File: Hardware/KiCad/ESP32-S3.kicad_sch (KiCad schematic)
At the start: 32 parts, among them J1 UJ20-C-H-G-SMT-1-P16-TR, J4 RJ45, J5 Conn_TagConnect_TC2030-NL_ESP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, U1 ESP32-S3-WROOM-1, U5 WE-TVS-82400102, U7 AP7333-33SRG-7

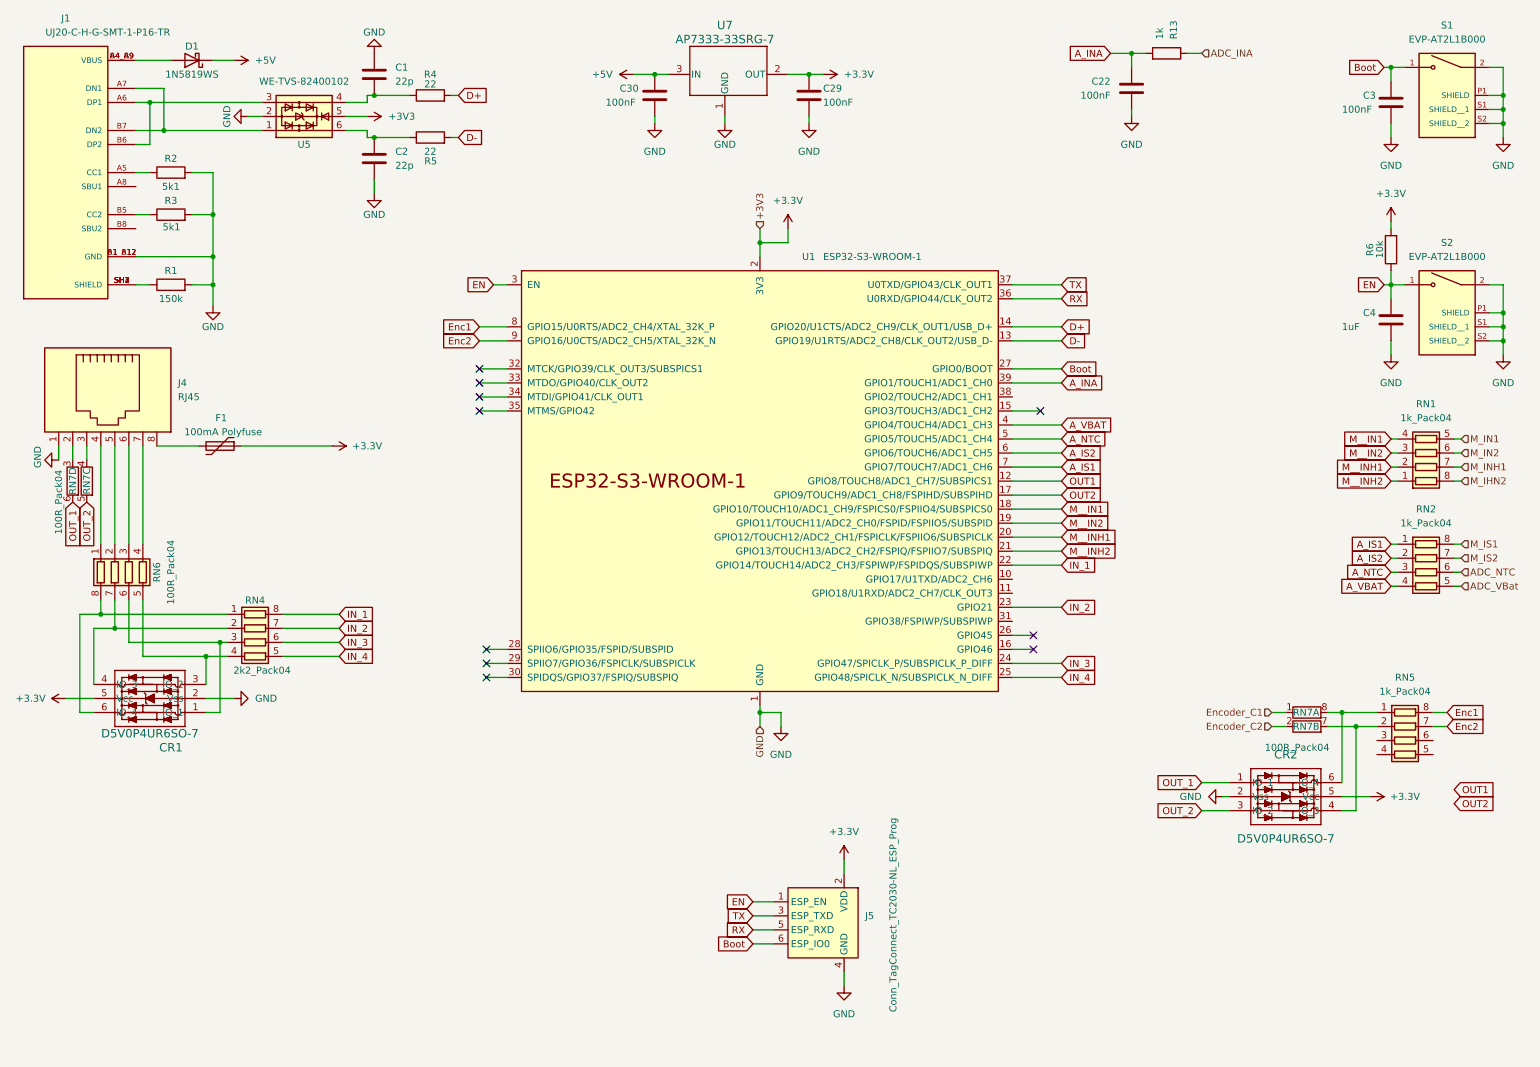
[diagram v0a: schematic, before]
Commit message: routing
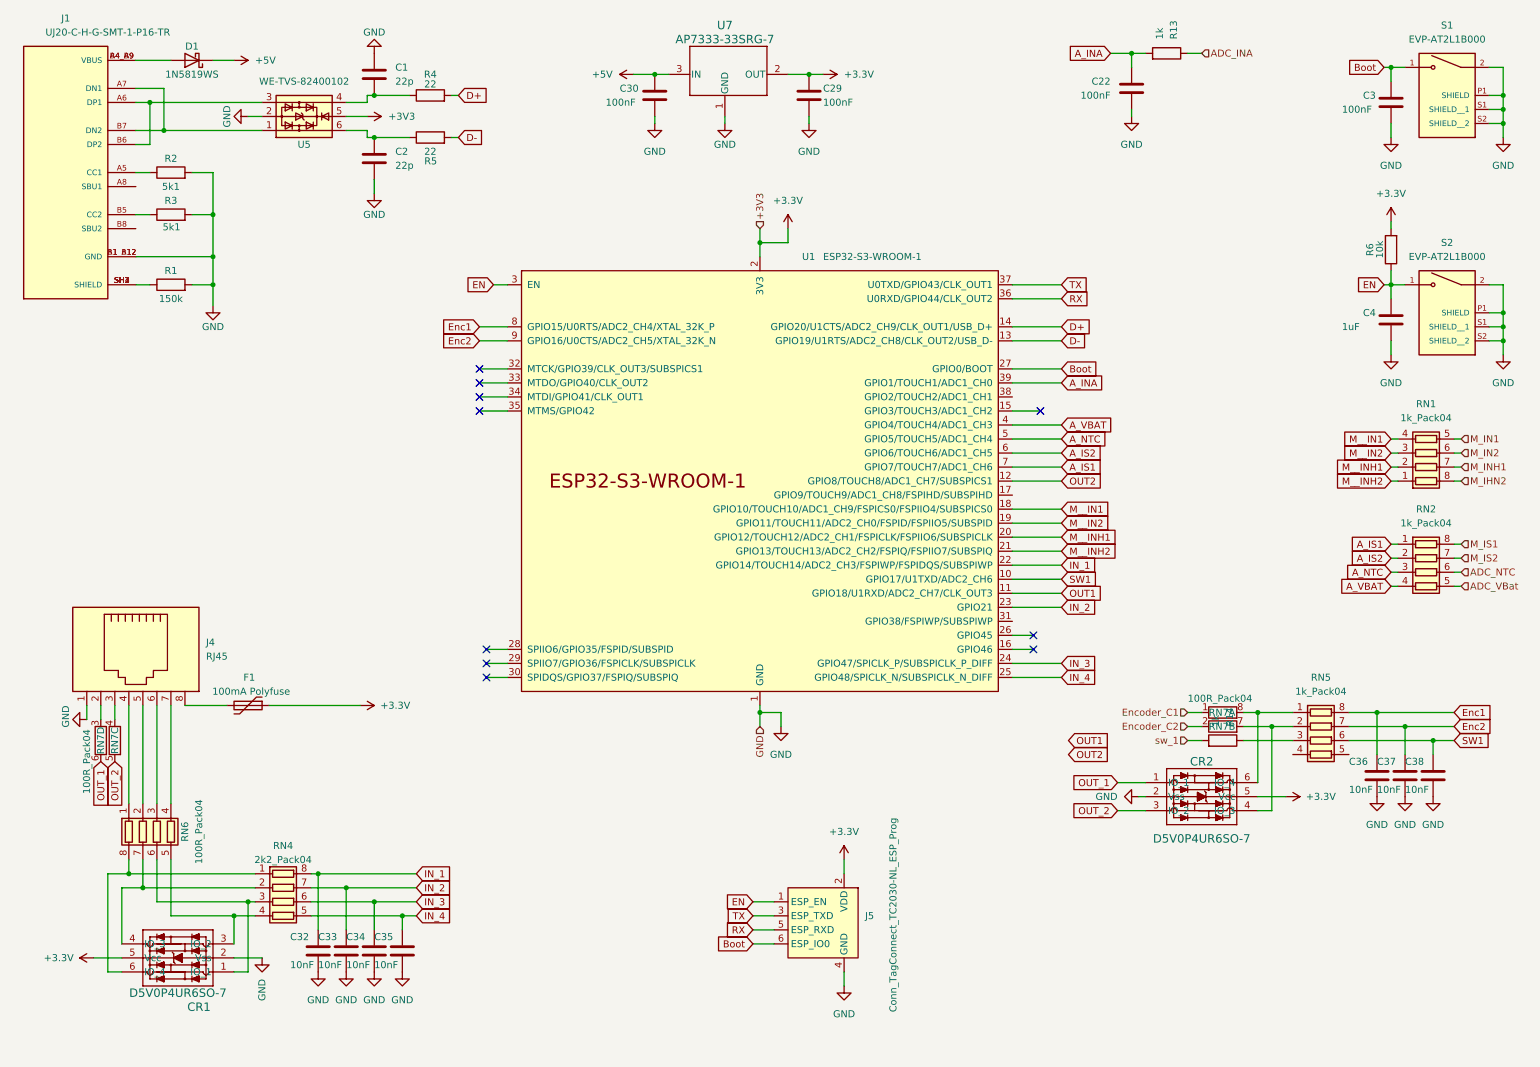
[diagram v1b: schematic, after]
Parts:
- added C32, C33, C34, C35, C36, C37, C38: 10nF, Capacitor_SMD:C_0603_1608Metric, symbol Device:C
- added R14: 1k, Resistor_SMD:R_0603_1608Metric, symbol Device:R
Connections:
- net Enc1: now also C36.1
- net Enc2: now also C37.1
- net GND: now also C32.2, C33.2, C34.2, C35.2, C36.2, C37.2, C38.2
- net IN_1: now also C32.1
- net IN_2: now also C33.1
- net IN_3: now also C34.1
- net IN_4: now also C35.1
- net OUT1: now also U1.11 (GPIO18/U1RXD/ADC2_CH7/CLK_OUT3); no longer U1.12 (GPIO8/TOUCH8/ADC1_CH7/SUBSPICS1)
- net OUT2: now also U1.12 (GPIO8/TOUCH8/ADC1_CH7/SUBSPICS1); no longer U1.17 (GPIO9/TOUCH9/ADC1_CH8/FSPIHD/SUBSPIHD)
- net SW1: now reaches U1.10 (GPIO17/U1TXD/ADC2_CH6)
- net SW1: now also RN5.6 (R3.2), C38.1
- net at RN5.3 (R3.1): now also R14.1
- new net sw_1: R14.2
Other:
- moved on the sheet: CR1, CR2, F1, J4, RN4, RN5, RN6, RN7A, RN7B, RN7C, RN7D

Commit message: PCB mostly finished
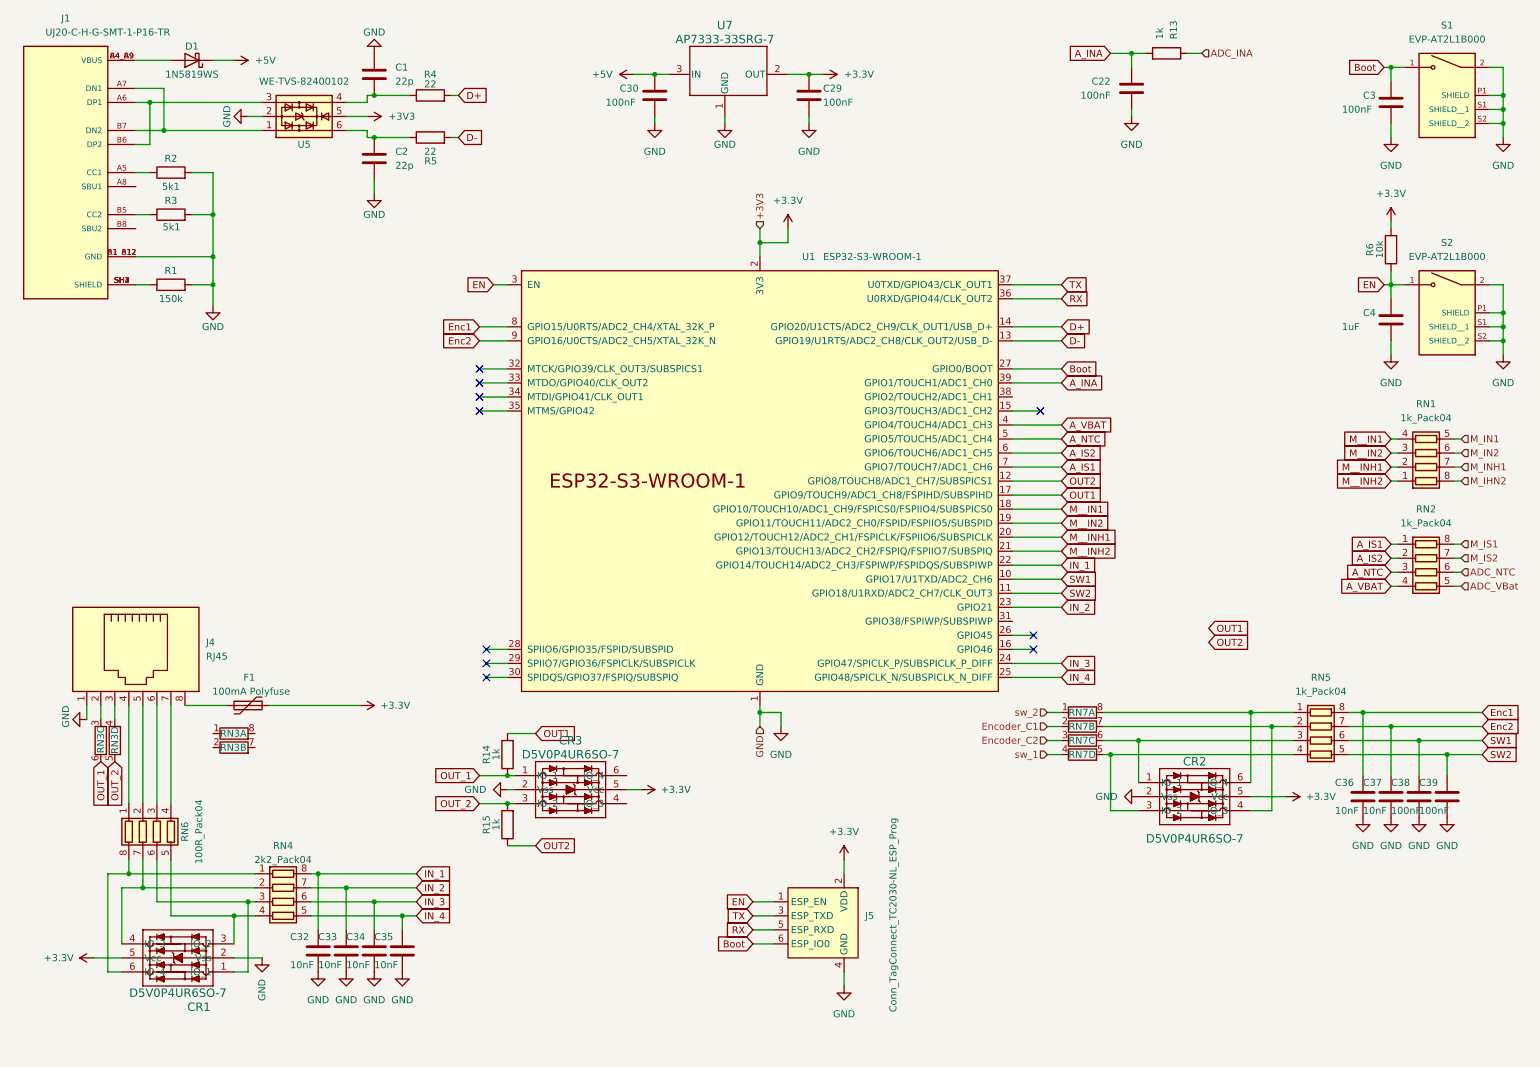
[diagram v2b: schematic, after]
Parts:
- added C39: 100nF, Capacitor_SMD:C_0603_1608Metric, symbol Device:C
- added CR3: D5V0P4UR6SO-7, BugWiper_lib:SOT26_DIO, symbol BugWiper_Lib:D5V0P4UR6SO-7
- added R15: 1k, Resistor_SMD:R_0603_1608Metric, symbol Device:R
- added RN3: 100R_Pack04, BugWiper_lib:BO_CAY16, symbol Device:R_Pack04_Split
- C38: value 10nF -> 100nF
- RN7: footprint Resistor_THT:R_Array_SIP8 -> BugWiper_lib:BO_CAY16
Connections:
- net +3.3V: now also CR3.5 (Vcc)
- net Encoder_C1: now also RN7.2 (R2.1); no longer RN7.1 (R1.1)
- net Encoder_C2: now also RN7.3 (R3.1); no longer RN7.2 (R2.1)
- net GND: now also C39.2, CR3.2 (Vss)
- net OUT1: now also R14.2, U1.17 (GPIO9/TOUCH9/ADC1_CH8/FSPIHD/SUBSPIHD); no longer U1.11 (GPIO18/U1RXD/ADC2_CH7/CLK_OUT3)
- net OUT2: now also R15.1
- net OUT_1: now also R14.1, CR3.1 (IO_1), RN3.6 (R3.2); no longer CR2.1 (IO_1), RN7.6 (R3.2)
- net OUT_2: now also CR3.3 (IO_2), R15.2, RN3.5 (R4.2); no longer CR2.3 (IO_2), RN7.5 (R4.2)
- net sw_1: now also RN7.4 (R4.1); no longer R14.2
- net at RN5.3 (R3.1): now also CR2.1 (IO_1), RN7.6 (R3.2); no longer R14.1
- net at J4.2: now also RN3.3 (R3.1); no longer RN7.3 (R3.1)
- net at J4.3: now also RN3.4 (R4.1); no longer RN7.4 (R4.1)
- net at RN5.4 (R4.1): now also CR2.3 (IO_2), RN7.5 (R4.2)
- net SW2: now reaches RN5.5 (R4.2)
- net SW2: now also U1.11 (GPIO18/U1RXD/ADC2_CH7/CLK_OUT3), C39.1
- new net sw_2: RN7.1 (R1.1)
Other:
- moved on the sheet: C36, C37, C38, CR2, RN7A, RN7B
